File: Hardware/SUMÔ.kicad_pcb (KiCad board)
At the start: 2 copper layers, 83.2 x 43.4 mm, 15 parts, among them SW1 SW_DPST_x2

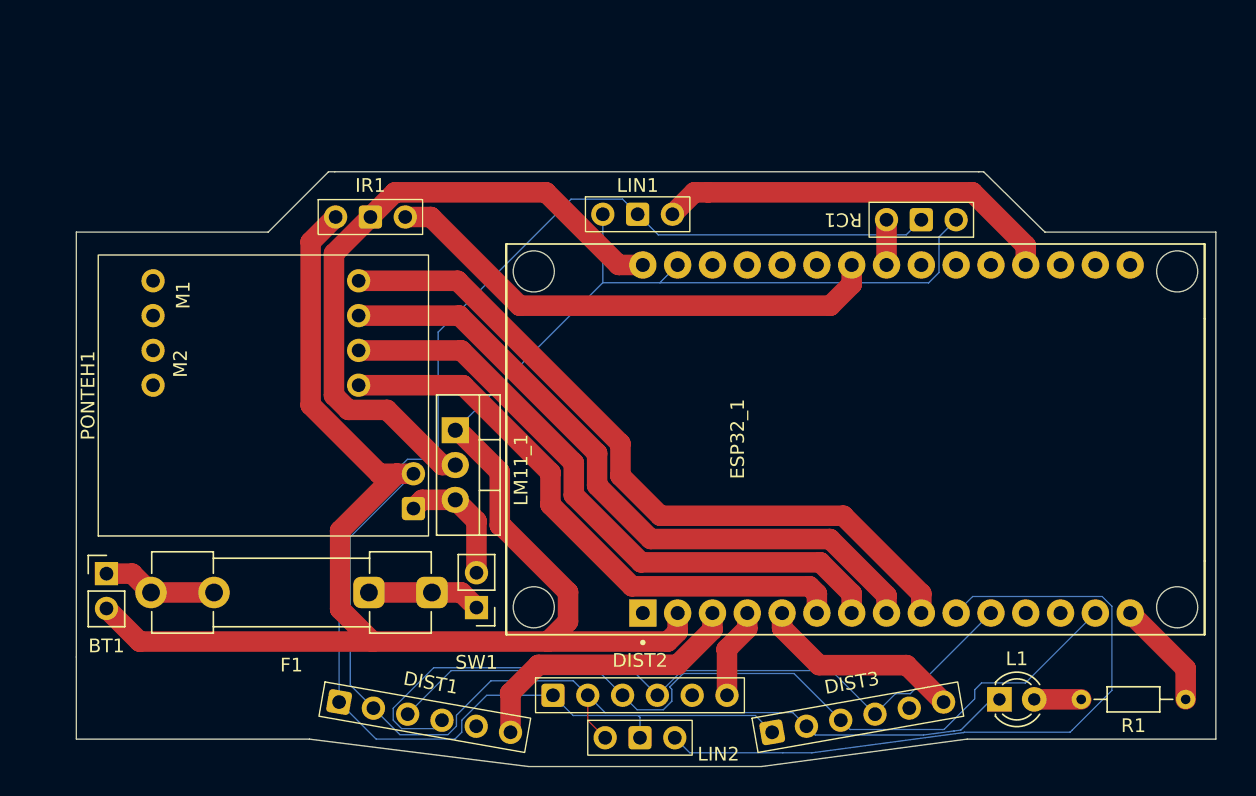
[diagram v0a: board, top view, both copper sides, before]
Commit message: V3: (circuito) update Hardware
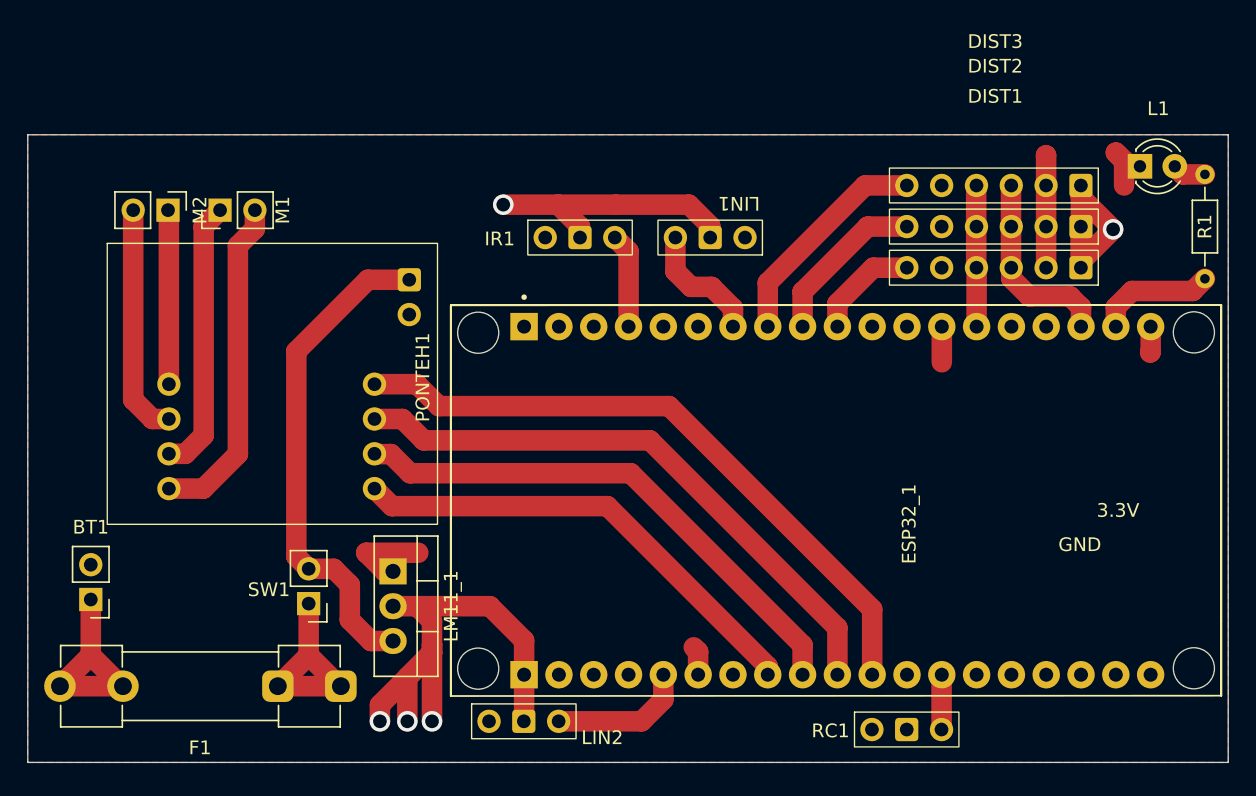
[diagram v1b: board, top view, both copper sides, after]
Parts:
- added M1: Motor_DC, Connector_PinHeader_2.54mm:PinHeader_1x02_P2.54mm_Vertical, F.Cu at (119.4, 55.7)
- added M2: Motor_DC, Connector_PinHeader_2.54mm:PinHeader_1x02_P2.54mm_Vertical, F.Cu at (115.6, 55.7)
- moved DIST1 56.8 mm to (175.9, 53.9), turned to 180 degrees
- moved DIST2 42.9 mm to (175.9, 56.9), turned to 180 degrees
- moved L1 40.2 mm to (186.6, 52.5)
- moved RC1 37.2 mm to (169.5, 93.6), turned to 0 degrees
- moved DIST3 34.3 mm to (175.9, 59.9), turned to 180 degrees
- moved R1 30.7 mm to (191.3, 60.7), turned to 90 degrees
- moved IR1 15.4 mm to (145.7, 57.7)
- moved SW1 12.2 mm to (125.9, 84.4)
- moved LM11_1 11.3 mm to (132.1, 82.1)
- moved F1 9.53 mm to (128.2, 90.4)
- moved LIN2 8.56 mm to (141.6, 93.0)
- moved LIN1 5.56 mm to (155.2, 57.7), turned to 180 degrees
- moved PONTEH1 5.24 mm to (115.7, 78.6)
- moved ESP32_1 4.66 mm to (167.0, 76.9)
- moved BT1 2.21 mm to (110.0, 84.1), turned to 180 degrees
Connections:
- ESP32_1 pad 10: LIN_2 -> DIST_XSHUT_3
- ESP32_1 pad 11: DIST_SDA -> unconnected-(ESP32_1-G18-Pad11)
- ESP32_1 pad 13: unconnected-(ESP32_1-TX0-Pad13) -> GND
- ESP32_1 pad 14: DIST_SCL -> DIST_SDA
- ESP32_1 pad 15: LED -> unconnected-(ESP32_1-Pad15)
- ESP32_1 pad 17: unconnected-(ESP32_1-VP-Pad17) -> DIST_SCL
- ESP32_1 pad 18: unconnected-(ESP32_1-VN-Pad18) -> LED
- ESP32_1 pad 19: LIN_1 -> GND
- ESP32_1 pad 2: GND -> unconnected-(ESP32_1-SDC-Pad2)
- ESP32_1 pad 23: RC -> unconnected-(ESP32_1-Pad23)
- ESP32_1 pad 24: IR -> unconnected-(ESP32_1-G34-Pad24)
- ESP32_1 pad 26: unconnected-(ESP32_1-D14-Pad26) -> RC
- ESP32_1 pad 28: unconnected-(ESP32_1-D13-Pad28) -> PONTEH_1
- ESP32_1 pad 29: GND -> PONTEH_2
- ESP32_1 pad 3: DIST_XSHUT_1 -> unconnected-(ESP32_1-SDI-Pad3)
- ESP32_1 pad 30: VCC 3.3v -> PONTEH_3
- ESP32_1 pad 4: DIST_XSHUT_2 -> IR
- ESP32_1 pad 5: DIST_XSHUT_3 -> unconnected-(ESP32_1-G2-Pad5)
- ESP32_1 pad 6: PONTEH_1 -> unconnected-(ESP32_1-G0-Pad6)
- ESP32_1 pad 7: PONTEH_2 -> LIN_1
- ESP32_1 pad 8: PONTEH_3 -> DIST_XSHUT_1
- ESP32_1 pad 9: PONTEH_4 -> DIST_XSHUT_2
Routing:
- net GND: track 228.7 -> 26.0 mm
- net VCC 3.3v: track 160.5 -> 71.9 mm, vias 0 -> 5
- net DIST_SCL: track 60.2 -> 14.1 mm
- net DIST_SDA: track 55.7 -> 9.80 mm
- net LIN_2: track 52.0 -> 10.1 mm
- net IR: track 37.3 -> 6.91 mm
- net VCC 12v: track 9.28 -> 36.5 mm
- net Net-(M1--): track 0.00 -> 24.4 mm
- net LIN_1: track 29.5 -> 9.12 mm
- net Net-(M1-+): track 0.00 -> 20.0 mm
- net PONTEH_4: track 53.3 -> 34.7 mm
- net Net-(M2--): track 0.00 -> 17.0 mm
- net Net-(M2-+): track 0.00 -> 12.7 mm
- net PONTEH_3: track 49.6 -> 39.2 mm
- net DIST_XSHUT_3: track 15.1 -> 7.84 mm
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- added copper zone on F.Cu, net GND
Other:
- board size 83.2 x 43.4 mm -> 87.6 x 45.8 mm
- board text added: "3.3V"
- board text added: "GND"
- board text removed: "M1"
- board text removed: "M2"
